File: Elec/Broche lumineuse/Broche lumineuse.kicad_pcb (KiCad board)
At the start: 2 copper layers, 40 x 10.4 mm, 30 parts, among them J1 USB_B_Micro, J2 Conn_01x02, J3 Conn_01x02, J4 Conn_01x03, J5 Conn_01x06_Male, Q1 PMV20XNEAR, Q2 DMN2215UDM-7, U1 ATtiny85V-10MU, U2 MMA8453Q, U3 MCP1700-2502E_SOT23, U4 MCP73831-2-OT, U6 SN74LVC1T45DBV, U7 BQ29707DSER

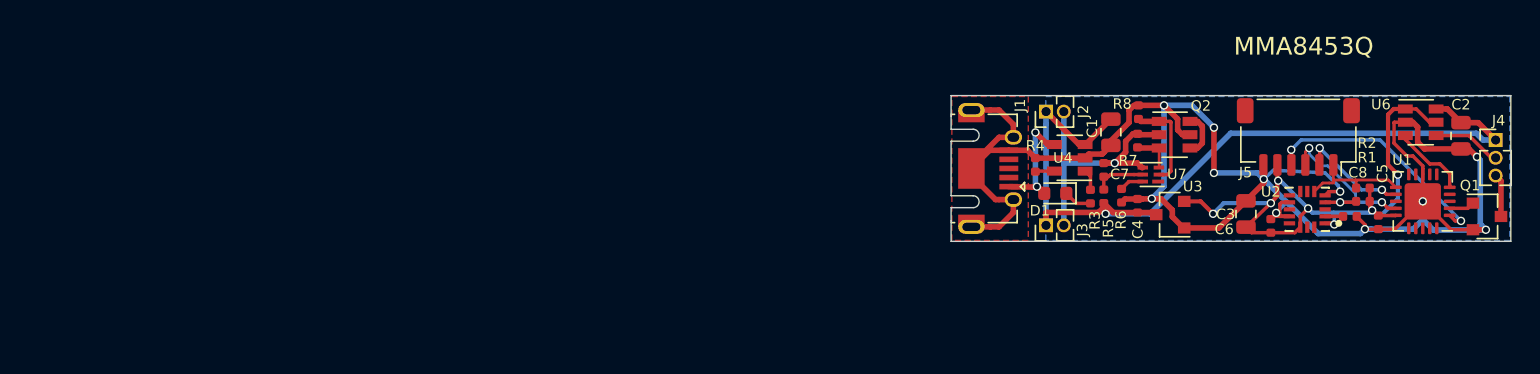
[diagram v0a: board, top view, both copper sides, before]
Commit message: Maj schéma suivant tests sur rev.1; Maj temporaire du PCB
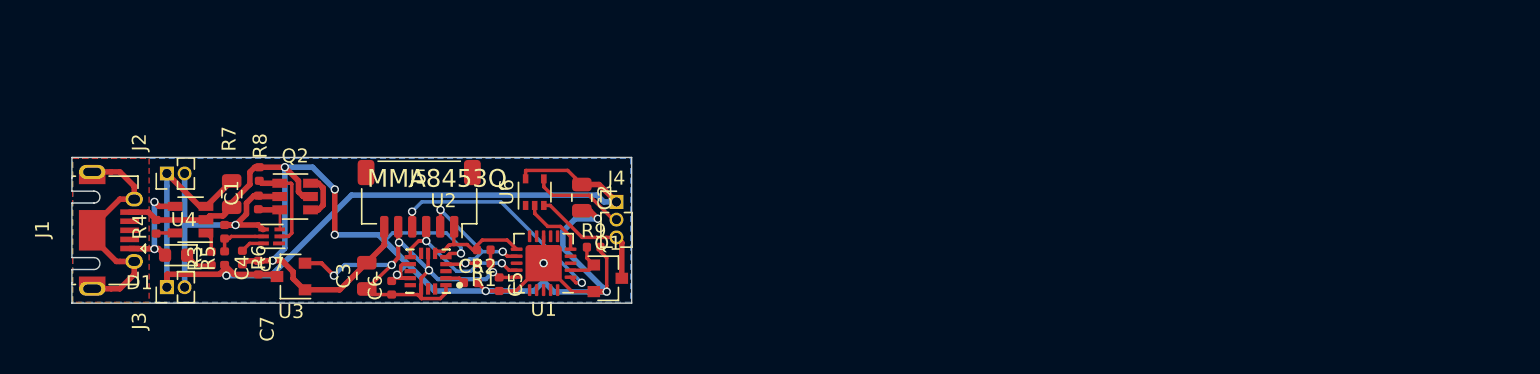
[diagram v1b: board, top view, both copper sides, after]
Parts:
- added R9: 56kR, Resistor_SMD:R_0402_1005Metric, F.Cu at (107.6, 99.6)
- U6: value SN74LVC1T45DBV -> SN74LV1T34DBVR; footprint Package_TO_SOT_SMD:SOT-23-6 -> Package_TO_SOT_SMD:SOT-353_SC-70-5
- moved U6 63.5 mm to (103.4, 95.7), turned to 90 degrees
- moved C8 63.0 mm to (98.8, 102.2)
- moved Q2 63.0 mm to (86.3, 96.0)
- moved C3 63.0 mm to (91.4, 101.7)
- moved C5 63.0 mm to (100.8, 102.3)
- moved C7 63.0 mm to (81.2, 98.5)
- moved J1 63.0 mm to (71.8, 98.4)
- moved J2 63.0 mm to (77.1, 94.4)
- moved J3 63.0 mm to (77.1, 102.5)
- moved J4 63.0 mm to (109.2, 96.4)
- moved Q1 63.0 mm to (108.6, 101.9)
- moved R4 63.0 mm to (76.3, 98.2)
- moved R5 63.0 mm to (81.2, 100.4)
- moved U3 63.0 mm to (86.0, 101.7)
- moved C2 63.0 mm to (106.7, 96.1)
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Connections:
- J1 pad 2: Net-(J1-Pad2) -> (no net)
- J1 pad 3: Net-(J1-Pad3) -> (no net)
- J1 pad 4: Net-(J1-Pad4) -> (no net)
- J1 pad 6: GND -> Net-(J1-Pad6)
- J4 pad 3: Net-(J4-Pad3) -> LED_GND
- J5 pad 2: /MISO -> SCL
- J5 pad 3: SCL -> INT0
- Q1 pad 3: Net-(J4-Pad3) -> LED_GND
- U1 pad 10: Net-(U1-Pad10) -> (no net)
- U1 pad 12: /MISO -> SCL
- U1 pad 13: Net-(U1-Pad13) -> (no net)
- U1 pad 14: SCL -> INT0
- U1 pad 16: Net-(U1-Pad16) -> (no net)
- U1 pad 17: Net-(U1-Pad17) -> (no net)
- U1 pad 18: Net-(U1-Pad18) -> (no net)
- U1 pad 19: Net-(U1-Pad19) -> (no net)
- U1 pad 20: Net-(U1-Pad20) -> (no net)
- U1 pad 3: Net-(U1-Pad3) -> (no net)
- U1 pad 4: Net-(U1-Pad4) -> (no net)
- U1 pad 6: Net-(U1-Pad6) -> (no net)
- U1 pad 7: Net-(U1-Pad7) -> (no net)
- U1 pad 9: Net-(U1-Pad9) -> (no net)
- U2 pad 11: Net-(U2-Pad11) -> (no net)
- U2 pad 13: Net-(U2-Pad13) -> (no net)
- U2 pad 15: Net-(U2-Pad15) -> (no net)
- U2 pad 16: Net-(U2-Pad16) -> (no net)
- U2 pad 3: Net-(U2-Pad3) -> (no net)
- U2 pad 7: Net-(U2-Pad7) -> +2V5
- U2 pad 8: Net-(U2-Pad8) -> (no net)
- U2 pad 9: Net-(U2-Pad9) -> INT0
- U6 pad 1: +2V5 -> (no net)
- U6 pad 2: GND -> LED_CMD
- U6 pad 3: LED_CMD -> LED_GND
- U6 pad 5: +2V5 -> +BATT
- U7 pad 1: Net-(U7-Pad1) -> (no net)
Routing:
- net GND: track 132.7 -> 109.8 mm, vias 11 -> 10
- net Net-(J1-Pad6): track 0.00 -> 17.0 mm
- net INT0: track 0.00 -> 10.8 mm, vias 0 -> 2
- net +2V5: track 43.6 -> 34.0 mm, vias 7 -> 5
- net LED_GND: track 0.00 -> 9.22 mm
- net /MISO: track 8.03 -> 0.00 mm, vias 2 -> 0
- net Net-(J4-Pad3): track 3.08 -> 0.00 mm
- net +BATT: track 60.5 -> 63.3 mm
- net LED_INPUT: track 4.91 -> 6.74 mm
- net LED_PWR: track 1.82 -> 3.29 mm
- net SCL: track 13.3 -> 11.9 mm
- net LED_CMD: track 5.44 -> 4.72 mm
- net VBUS: track 8.36 -> 7.71 mm
- added copper zone on F.Cu, net Net-(J1-Pad6)
- removed copper zone on F.Cu, net GND
